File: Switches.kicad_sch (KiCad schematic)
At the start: 26 parts

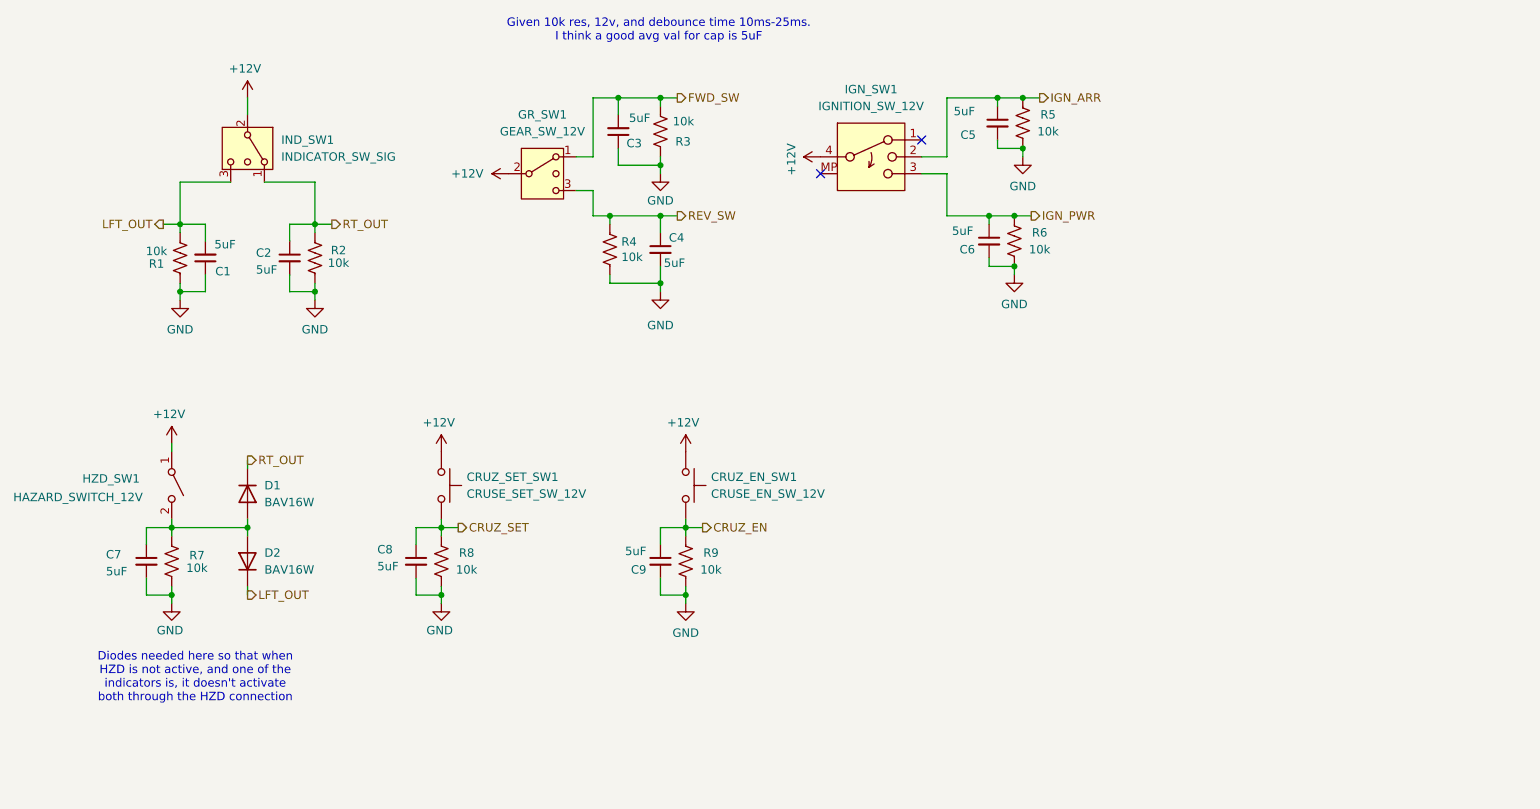
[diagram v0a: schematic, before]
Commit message: Made pretty
Fixed a few things up and made it pretty.
Still need to double check a few things and assign all footprints
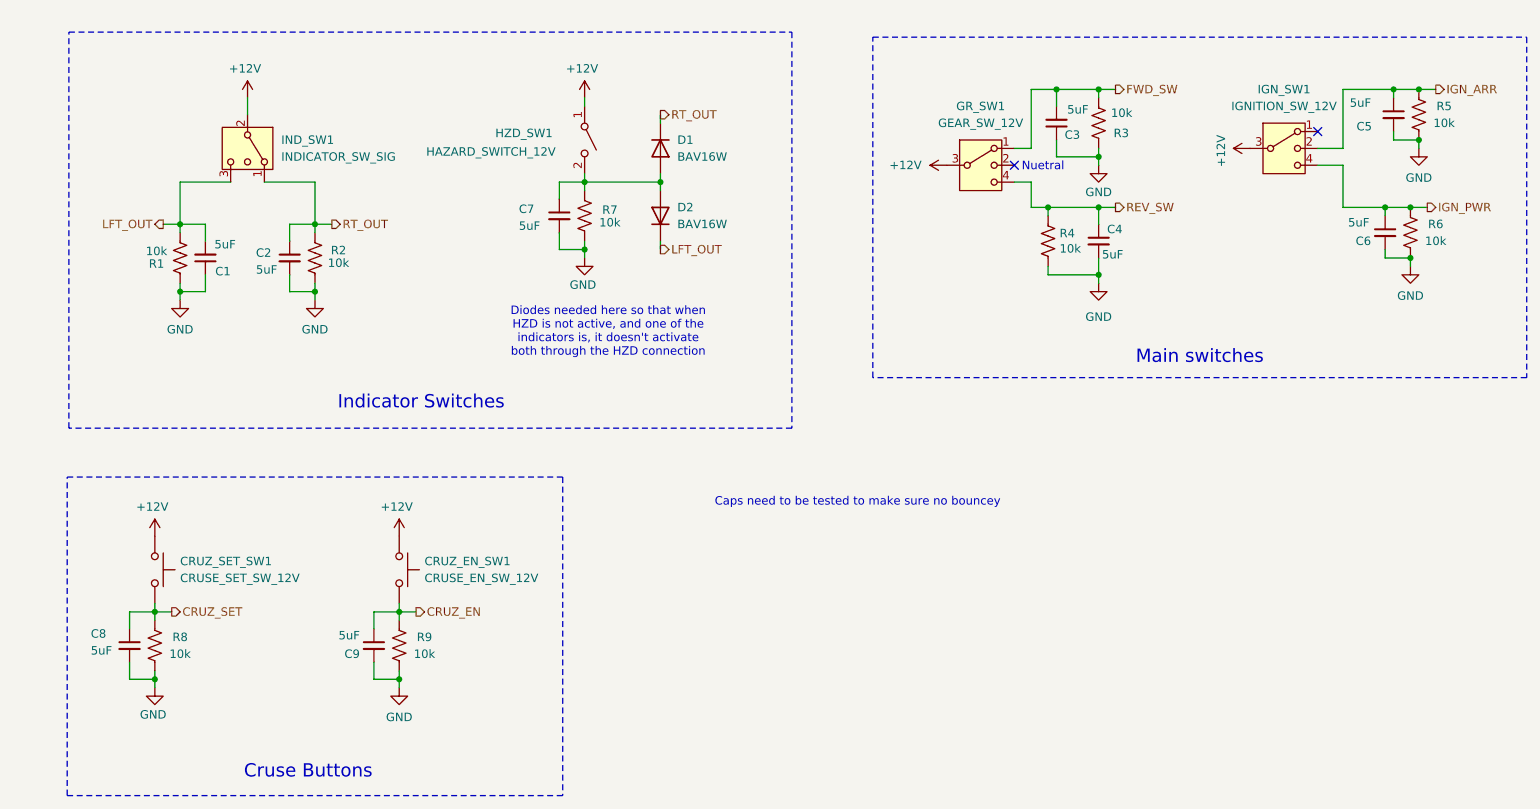
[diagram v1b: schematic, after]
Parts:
- GR_SW1: symbol Switch:SW_SPDT_MSM -> Switch:SW_SP3T
- IGN_SW1: symbol Switch:SW_Rotary_1x3_MP -> Switch:SW_SP3T
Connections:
- net +12V: now also GR_SW1.3, IGN_SW1.3; no longer GR_SW1.2 (3), IGN_SW1.4
- net IGN_PWR: now also IGN_SW1.4; no longer IGN_SW1.3
- net REV_SW: now also GR_SW1.4; no longer GR_SW1.3 (4)
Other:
- note added: "Caps need to be tested to make sure no bouncey"
- note added: "Cruse Buttons"
- note added: "Indicator Switches"
- note added: "Main switches"
- note added: "Nuetral"
- note removed: "Given 10k res, 12v, and debounce time 10ms-25ms. I think a good avg val for cap is 5uF"
- moved on the sheet: C3, C4, C5, C6, C7, C8, C9, CRUZ_EN_SW1, CRUZ_SET_SW1, D1, D2, HZD_SW1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
